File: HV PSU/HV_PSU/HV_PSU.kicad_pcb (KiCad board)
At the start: 2 copper layers, 106 parts, among them J1 Screw_Terminal_01x07, J10 MountingHole_Pad, J11 MountingHole_Pad, J12 MountingHole_Pad, J13 MountingHole_Pad, J2 MountingHole_Pad, J3 MountingHole_Pad, J4 MountingHole_Pad, J5 MountingHole_Pad, J6 MountingHole_Pad, J7 MountingHole_Pad, J8 MountingHole_Pad, J9 MountingHole_Pad, Q1 2N7002, Q2 IRFS4227, Q3 IRFS4227, U1 L7812, U2 TPS2814D

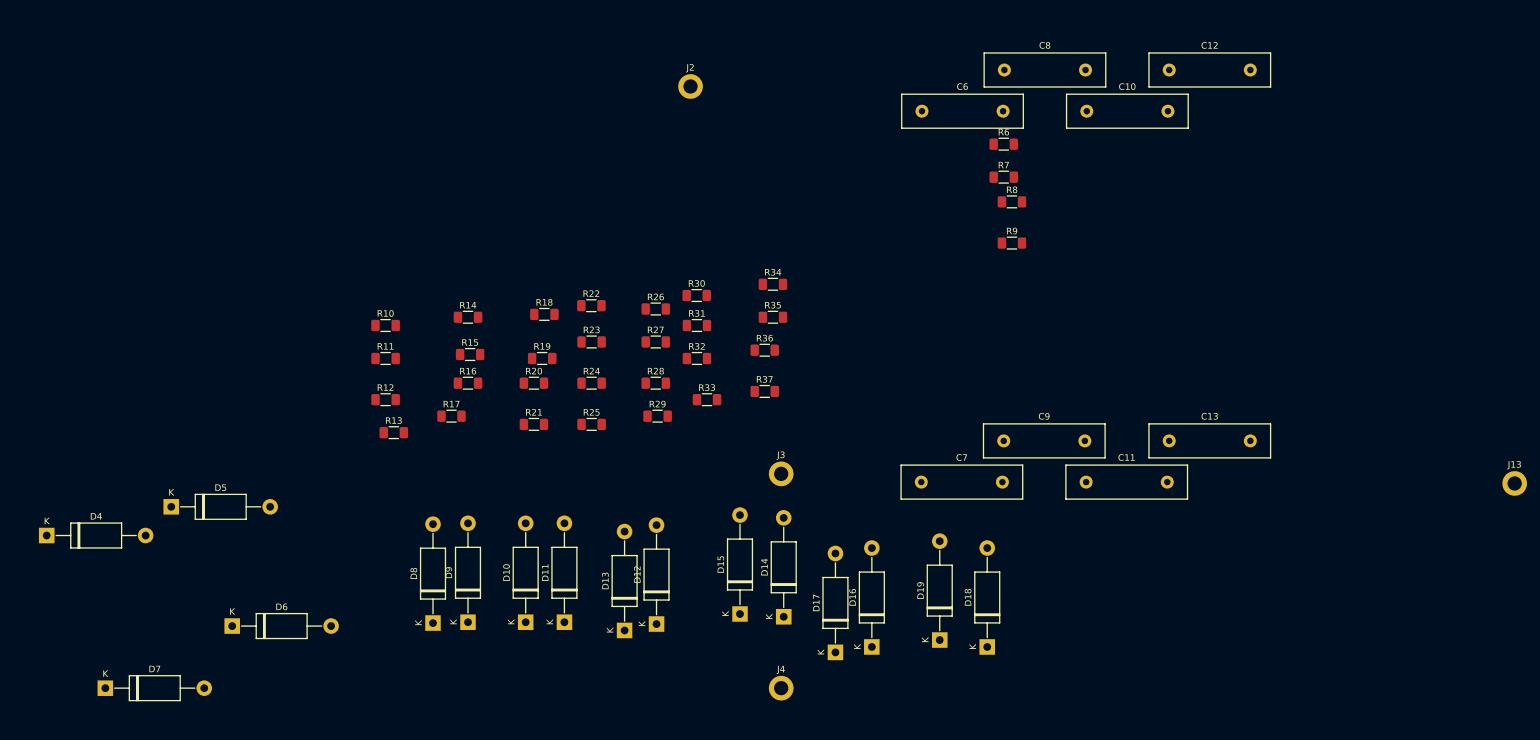
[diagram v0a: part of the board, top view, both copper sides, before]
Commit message: Some PCB placement
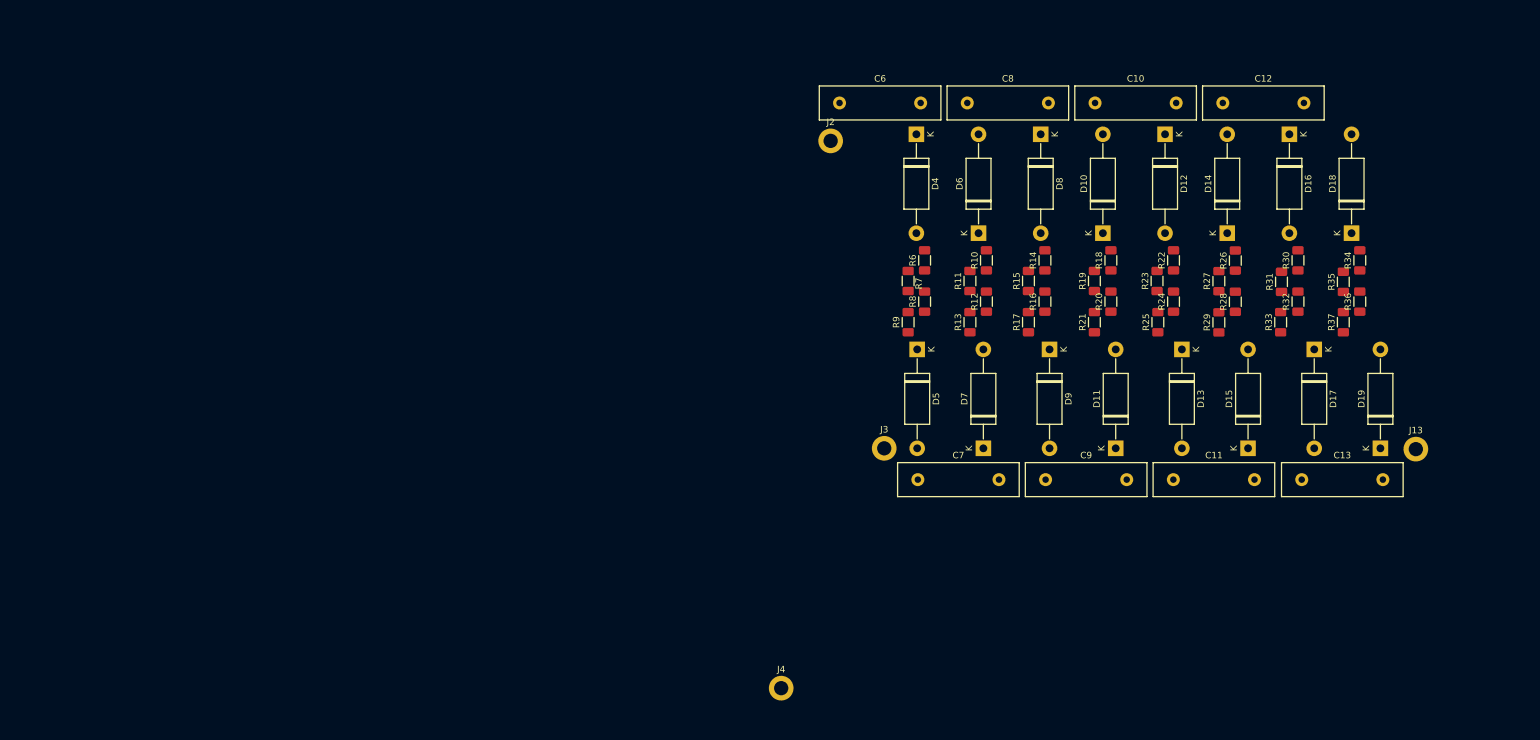
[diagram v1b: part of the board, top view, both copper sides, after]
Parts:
- moved D4 147.6 mm to (254.5, 95.0), turned to -90 degrees
- moved D7 140.2 mm to (264.8, 143.4), turned to 90 degrees
- moved D6 130.0 mm to (264.1, 110.2), turned to 90 degrees
- moved D8 120.2 mm to (273.7, 95.0), turned to -90 degrees
- moved D5 117.5 mm to (254.6, 128.1), turned to -90 degrees
- moved D12 108.8 mm to (292.8, 95.0), turned to -90 degrees
- moved D10 107.3 mm to (283.2, 110.2)
- moved D16 101.9 mm to (312.0, 95.0), turned to -90 degrees
- moved D9 99.0 mm to (275.0, 128.1), turned to -90 degrees
- moved D13 96.2 mm to (295.4, 128.1), turned to -90 degrees
- moved R12 93.8 mm to (265.3, 120.8), turned to 90 degrees
- moved R10 93.1 mm to (265.3, 114.4), turned to 90 degrees
- moved R32 93.0 mm to (313.3, 120.8), turned to 90 degrees
- moved R30 92.8 mm to (313.3, 114.4), turned to 90 degrees
- moved R36 92.0 mm to (322.8, 120.8), turned to 90 degrees
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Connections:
- D10 pad 1: Net-(D10-Pad1) -> Net-(R18-Pad2)
- D10 pad 2: Net-(D10-Pad2) -> Net-(C10-Pad1)
- D11 pad 2: Net-(D10-Pad1) -> Net-(D11-Pad2)
- D12 pad 1: Net-(D12-Pad1) -> Net-(C10-Pad2)
- D12 pad 2: Net-(D12-Pad2) -> Net-(R22-Pad2)
- D13 pad 1: Net-(D12-Pad2) -> Net-(D13-Pad1)
- D14 pad 1: Net-(D14-Pad1) -> Net-(R26-Pad2)
- D14 pad 2: Net-(D14-Pad2) -> Net-(C10-Pad2)
- D15 pad 2: Net-(D14-Pad1) -> Net-(D15-Pad2)
- D16 pad 1: Net-(D16-Pad1) -> Net-(C12-Pad2)
- D17 pad 1: Net-(D16-Pad2) -> Net-(D17-Pad1)
- D18 pad 1: Net-(D18-Pad1) -> Net-(R34-Pad2)
- D18 pad 2: Net-(D18-Pad2) -> Net-(C12-Pad2)
- D19 pad 2: Net-(D18-Pad1) -> Net-(R37-Pad1)
- D4 pad 1: Net-(D4-Pad1) -> Net-(C6-Pad2)
- D4 pad 2: Net-(D4-Pad2) -> Net-(R6-Pad2)
- D5 pad 1: Net-(D4-Pad2) -> Net-(D5-Pad1)
- D6 pad 2: Net-(D6-Pad2) -> Net-(C6-Pad2)
- D7 pad 2: Net-(D6-Pad1) -> Net-(D7-Pad2)
- D8 pad 1: Net-(D8-Pad1) -> Net-(C10-Pad1)
- D8 pad 2: Net-(D8-Pad2) -> Net-(R14-Pad2)
- D9 pad 1: Net-(D8-Pad2) -> Net-(D9-Pad1)
- R10 pad 2: Net-(C6-Pad2) -> Net-(D6-Pad1)
- R13 pad 1: Net-(D6-Pad2) -> Net-(D7-Pad2)
- R14 pad 2: Net-(C10-Pad1) -> Net-(R14-Pad2)
- R17 pad 1: Net-(D8-Pad1) -> Net-(D9-Pad1)
- R18 pad 2: Net-(C10-Pad1) -> Net-(R18-Pad2)
- R21 pad 1: Net-(D10-Pad2) -> Net-(D11-Pad2)
- R22 pad 2: Net-(C10-Pad2) -> Net-(R22-Pad2)
- R25 pad 1: Net-(D12-Pad1) -> Net-(D13-Pad1)
- R26 pad 2: Net-(C10-Pad2) -> Net-(R26-Pad2)
- R29 pad 1: Net-(D14-Pad2) -> Net-(D15-Pad2)
- R30 pad 2: Net-(C12-Pad2) -> Net-(D16-Pad2)
- R33 pad 1: Net-(D16-Pad1) -> Net-(D17-Pad1)
- R34 pad 2: Net-(C12-Pad2) -> Net-(R34-Pad2)
- R37 pad 1: Net-(D18-Pad2) -> Net-(R37-Pad1)
- R6 pad 2: Net-(C6-Pad2) -> Net-(R6-Pad2)
- R9 pad 1: Net-(D4-Pad1) -> Net-(D5-Pad1)
